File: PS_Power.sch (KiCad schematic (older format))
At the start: 17 parts, among them U28 MPM3840GQV-Z, U29 MPM3810AGQB-Z

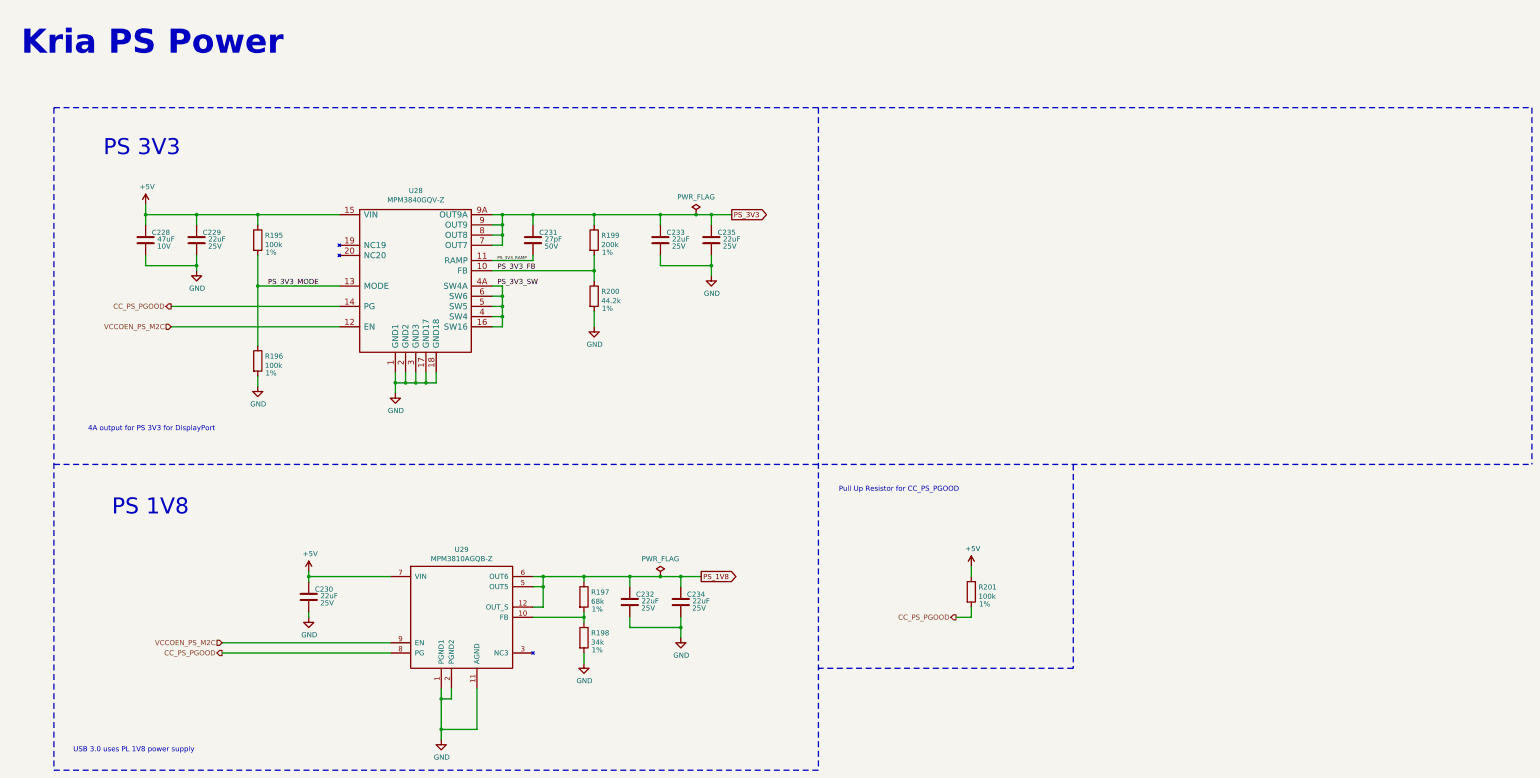
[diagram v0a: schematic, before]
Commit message: Update May --> See Update Note
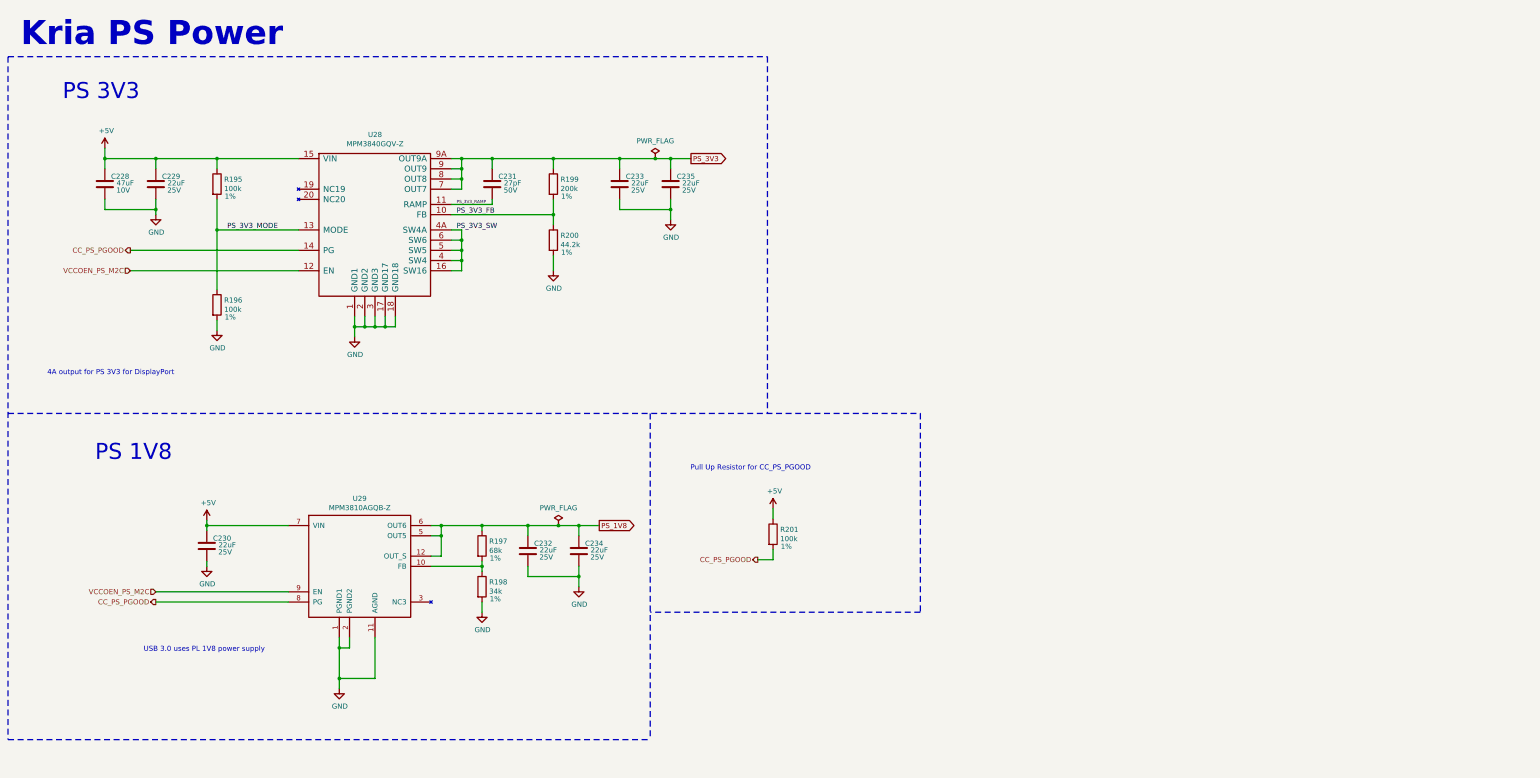
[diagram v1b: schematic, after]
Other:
- moved on the sheet: C228, C229, C230, C231, C232, C233, C234, C235, R195, R196, R197, R198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
